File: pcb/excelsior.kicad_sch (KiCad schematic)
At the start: 10 parts, among them J1 USB_Hub4_FDD, J2 USB_Hub3, J3 USB_Hub2, J4 Conn_01x40_Socket, P1 Host_Port, P2 Left_Peripheral, P3 Right_Peripheral, U1 kb2040, U2 MCP23017_SO, U3 CH334R

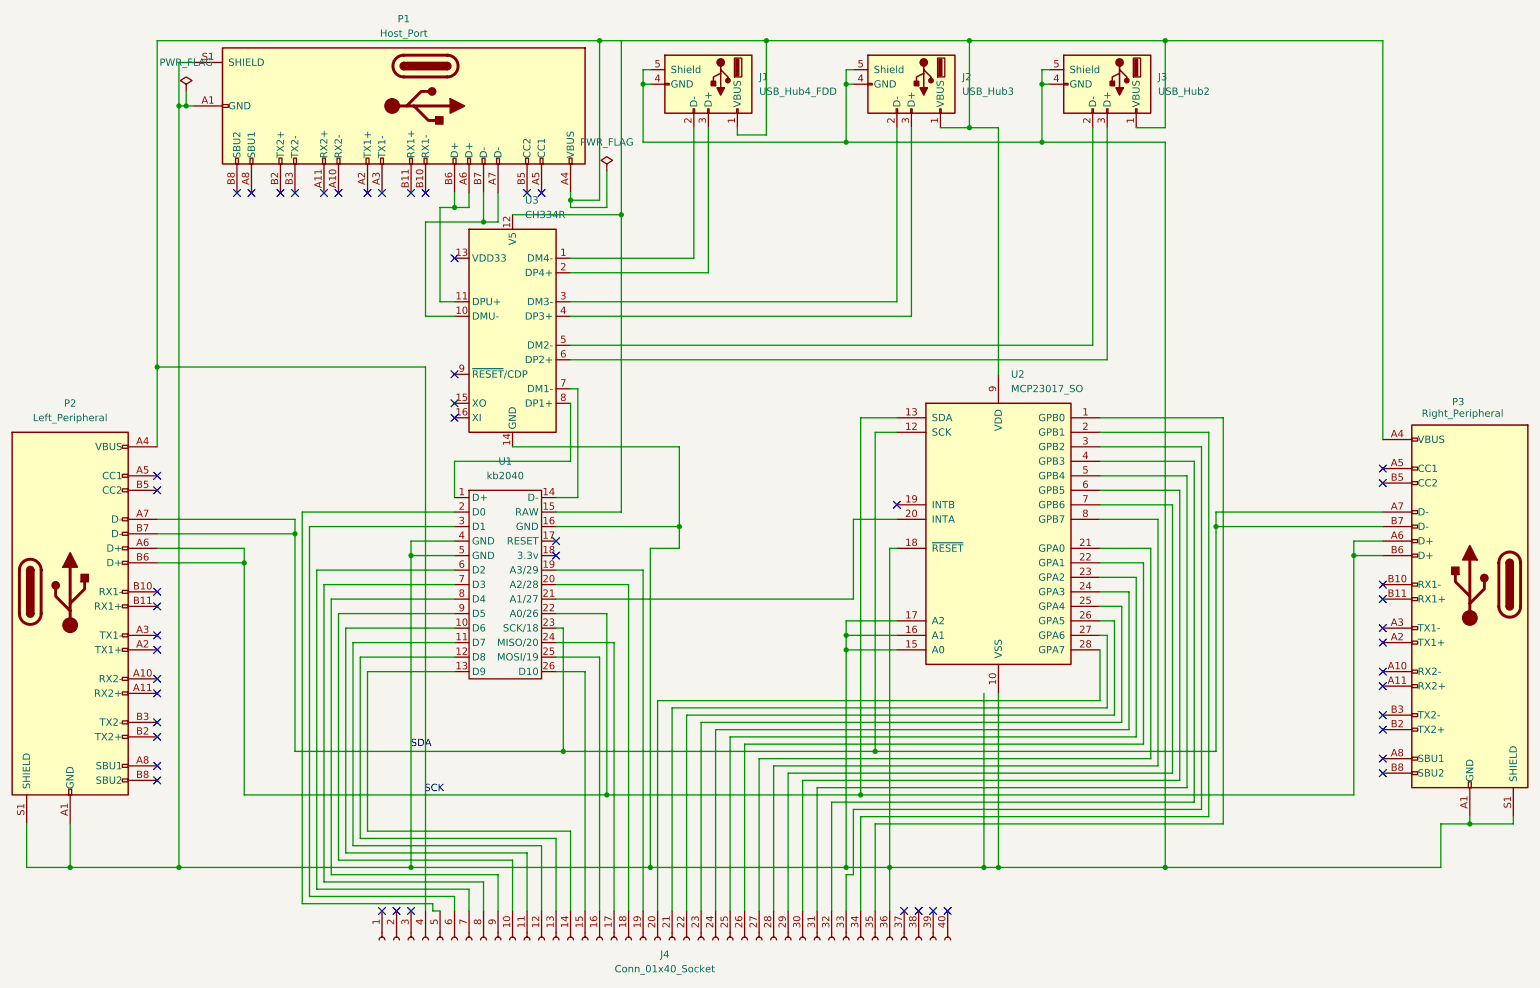
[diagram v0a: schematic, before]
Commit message: Continue work on PCB design.
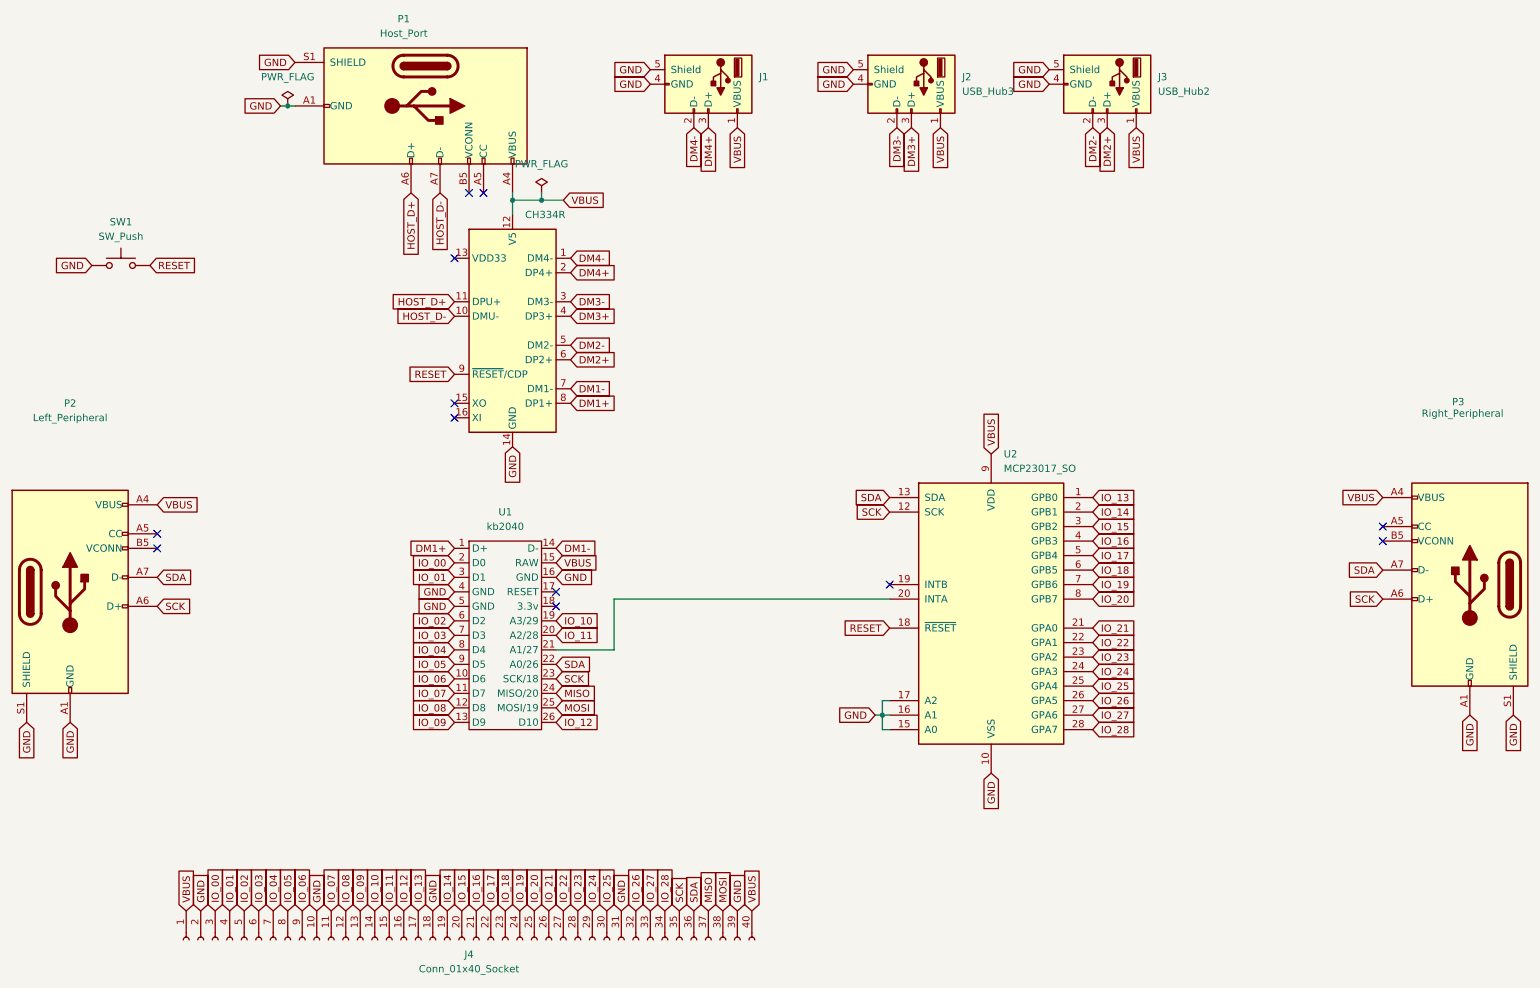
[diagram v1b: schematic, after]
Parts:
- added SW1: SW_Push, Button_Switch_SMD:SW_SPST_EVPBF, symbol Switch:SW_Push
- J1, J2, J3: footprint Connector_USB:USB_A_TE_292303-7_Horizontal -> Connector_USB:USB_A_Molex_67643_Horizontal
- P1, P2, P3: footprint Connector_USB:USB_C_Receptacle_Molex_105450-0101 -> Connector_USB:USB_C_Receptacle_GCT_USB4085; symbol Connector:USB_C_Receptacle -> Connector:USB_C_Plug_USB2.0
- U2: footprint Package_SO:SOIC-28W_7.5x17.9mm_P1.27mm -> Package_DIP:DIP-28_W7.62mm; symbol Interface_Expansion:MCP23017_SO -> Interface_Expansion:MCP23017_SP
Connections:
- net VBUS: now reaches J1.1 (VBUS), J2.1 (VBUS), J3.1 (VBUS), P1.A4 (VBUS), P1.A9 (VBUS), P1.B4 (VBUS), P1.B9 (VBUS), P2.A4 (VBUS), P2.A9 (VBUS), P2.B4 (VBUS), P2.B9 (VBUS), P3.A4 (VBUS), P3.A9 (VBUS), P3.B4 (VBUS), P3.B9 (VBUS), U1.15 (RAW), U2.9 (VDD), U3.12 (V5)
- net VBUS: now also J4.1 (Pin_1), J4.40 (Pin_40); no longer J4.4 (Pin_4)
- net DM2-: now reaches J3.2 (D-), U3.5 (DM2-)
- net DM2+: now reaches J3.3 (D+), U3.6 (DP2+)
- net GND: now reaches J1.4 (GND), J1.5 (Shield), J2.4 (GND), J2.5 (Shield), J3.4 (GND), J3.5 (Shield), P1.A1 (GND), P1.A12 (GND), P1.B1 (GND), P1.B12 (GND), P1.S1 (SHIELD), P2.A1 (GND), P2.A12 (GND), P2.B1 (GND), P2.B12 (GND), P2.S1 (SHIELD), P3.A1 (GND), P3.A12 (GND), P3.B1 (GND), P3.B12 (GND), P3.S1 (SHIELD), U1.16 (GND), U1.4 (GND), U1.5 (GND), U2.10 (VSS), U2.15 (A0), U2.16 (A1), U2.17 (A2), U3.14 (GND)
- net GND: now also J4.10 (Pin_10), J4.18 (Pin_18), J4.2 (Pin_2), J4.31 (Pin_31), J4.39 (Pin_39), SW1.1; no longer J4.36 (Pin_36), U2.18 (~{RESET})
- net IO_13: now reaches U2.1 (GPB0)
- net IO_13: now also J4.17 (Pin_17); no longer J4.35 (Pin_35)
- net IO_14: now reaches U2.2 (GPB1)
- net IO_14: now also J4.19 (Pin_19); no longer J4.34 (Pin_34)
- net IO_21: now reaches U2.21 (GPA0)
- net IO_21: now also J4.26 (Pin_26); no longer J4.27 (Pin_27)
- net IO_22: now reaches U2.22 (GPA1)
- net IO_22: now also J4.27 (Pin_27); no longer J4.26 (Pin_26)
- net IO_20: now reaches J4.25 (Pin_25)
- net IO_20: now also U2.8 (GPB7); no longer U2.23 (GPA2)
- net IO_19: now reaches J4.24 (Pin_24)
- net IO_19: now also U2.7 (GPB6); no longer U2.24 (GPA3)
- net IO_18: now reaches J4.23 (Pin_23)
- net IO_18: now also U2.6 (GPB5); no longer U2.25 (GPA4)
- net IO_17: now reaches J4.22 (Pin_22)
- net IO_17: now also U2.5 (GPB4); no longer U2.26 (GPA5)
- net IO_16: now reaches J4.21 (Pin_21)
- net IO_16: now also U2.4 (GPB3); no longer U2.27 (GPA6)
- net IO_15: now reaches J4.20 (Pin_20)
- net IO_15: now also U2.3 (GPB2); no longer U2.28 (GPA7)
- net IO_27: now reaches J4.33 (Pin_33)
- net IO_27: now also U2.27 (GPA6); no longer U2.3 (GPB2)
- net IO_26: now reaches J4.32 (Pin_32)
- net IO_26: now also U2.26 (GPA5); no longer U2.4 (GPB3)
- net IO_25: now reaches J4.30 (Pin_30)
- net IO_25: now also U2.25 (GPA4); no longer U2.6 (GPB5)
- net IO_24: now reaches J4.29 (Pin_29)
- net IO_24: now also U2.24 (GPA3); no longer U2.7 (GPB6)
- net IO_23: now reaches J4.28 (Pin_28)
- net IO_23: now also U2.23 (GPA2); no longer U2.8 (GPB7)
- net DM4-: now reaches J1.2 (D-), U3.1 (DM4-)
- net HOST_D-: now reaches P1.A7 (D-), U3.10 (DMU-)
- net HOST_D-: no longer P1.B7 (D-)
- net HOST_D+: now reaches P1.A6 (D+), U3.11 (DPU+)
- net HOST_D+: no longer P1.B6 (D+)
- net DM4+: now reaches J1.3 (D+), U3.2 (DP4+)
- net DM3-: now reaches J2.2 (D-), U3.3 (DM3-)
- net DM3+: now reaches J2.3 (D+), U3.4 (DP3+)
- net DM1-: now reaches U1.14 (D-), U3.7 (DM1-)
- net DM1+: now reaches U1.1 (D+), U3.8 (DP1+)
- net RESET: now reaches U3.9 (~{RESET}/CDP)
- net RESET: now also U2.18 (~{RESET}), SW1.2
- net IO_06: now reaches U1.10 (D6)
- net IO_06: now also J4.9 (Pin_9); no longer J4.11 (Pin_11)
- net IO_07: now reaches U1.11 (D7)
- net IO_07: now also J4.11 (Pin_11); no longer J4.12 (Pin_12)
- net IO_08: now reaches U1.12 (D8)
- net IO_08: now also J4.12 (Pin_12); no longer J4.13 (Pin_13)
- net IO_09: now reaches U1.13 (D9)
- net IO_09: now also J4.13 (Pin_13); no longer J4.14 (Pin_14)
- net IO_10: now reaches U1.19 (A3/29)
- net IO_10: now also J4.14 (Pin_14); no longer J4.19 (Pin_19)
- net IO_00: now reaches U1.2 (D0)
- net IO_00: now also J4.3 (Pin_3); no longer J4.5 (Pin_5)
- net IO_11: now reaches U1.20 (A2/28)
- net IO_11: now also J4.15 (Pin_15); no longer J4.18 (Pin_18)
- net MISO: now reaches U1.24 (MISO/20)
- net MISO: now also J4.37 (Pin_37); no longer J4.17 (Pin_17)
- net IO_12: now reaches J4.16 (Pin_16)
- net IO_12: now also U1.26 (D10); no longer U1.25 (MOSI/19)
- net IO_01: now reaches U1.3 (D1)
- net IO_01: now also J4.4 (Pin_4); no longer J4.6 (Pin_6)
- net IO_02: now reaches U1.6 (D2)
- net IO_02: now also J4.5 (Pin_5); no longer J4.7 (Pin_7)
- net IO_03: now reaches U1.7 (D3)
- net IO_03: now also J4.6 (Pin_6); no longer J4.8 (Pin_8)
- net IO_04: now reaches U1.8 (D4)
- net IO_04: now also J4.7 (Pin_7); no longer J4.9 (Pin_9)
- net IO_05: now reaches U1.9 (D5)
- net IO_05: now also J4.8 (Pin_8); no longer J4.10 (Pin_10)
- net MOSI: now reaches J4.38 (Pin_38)
- net MOSI: now also U1.25 (MOSI/19)
- new net IO_28: J4.34 (Pin_34), U2.28 (GPA7)
- new net SCK: J4.35 (Pin_35), P2.A6 (D+), P3.A6 (D+), U1.23 (SCK/18), U2.12 (SCK)
- new net SDA: J4.36 (Pin_36), P2.A7 (D-), P3.A7 (D-), U1.22 (A0/26), U2.13 (SDA)
- no-connect marks 50 -> 12
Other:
- note removed: "SCK"
- note removed: "SDA"
- moved on the sheet: J4, U1, U2

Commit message: Continue work on PCBs, add Gerber files.
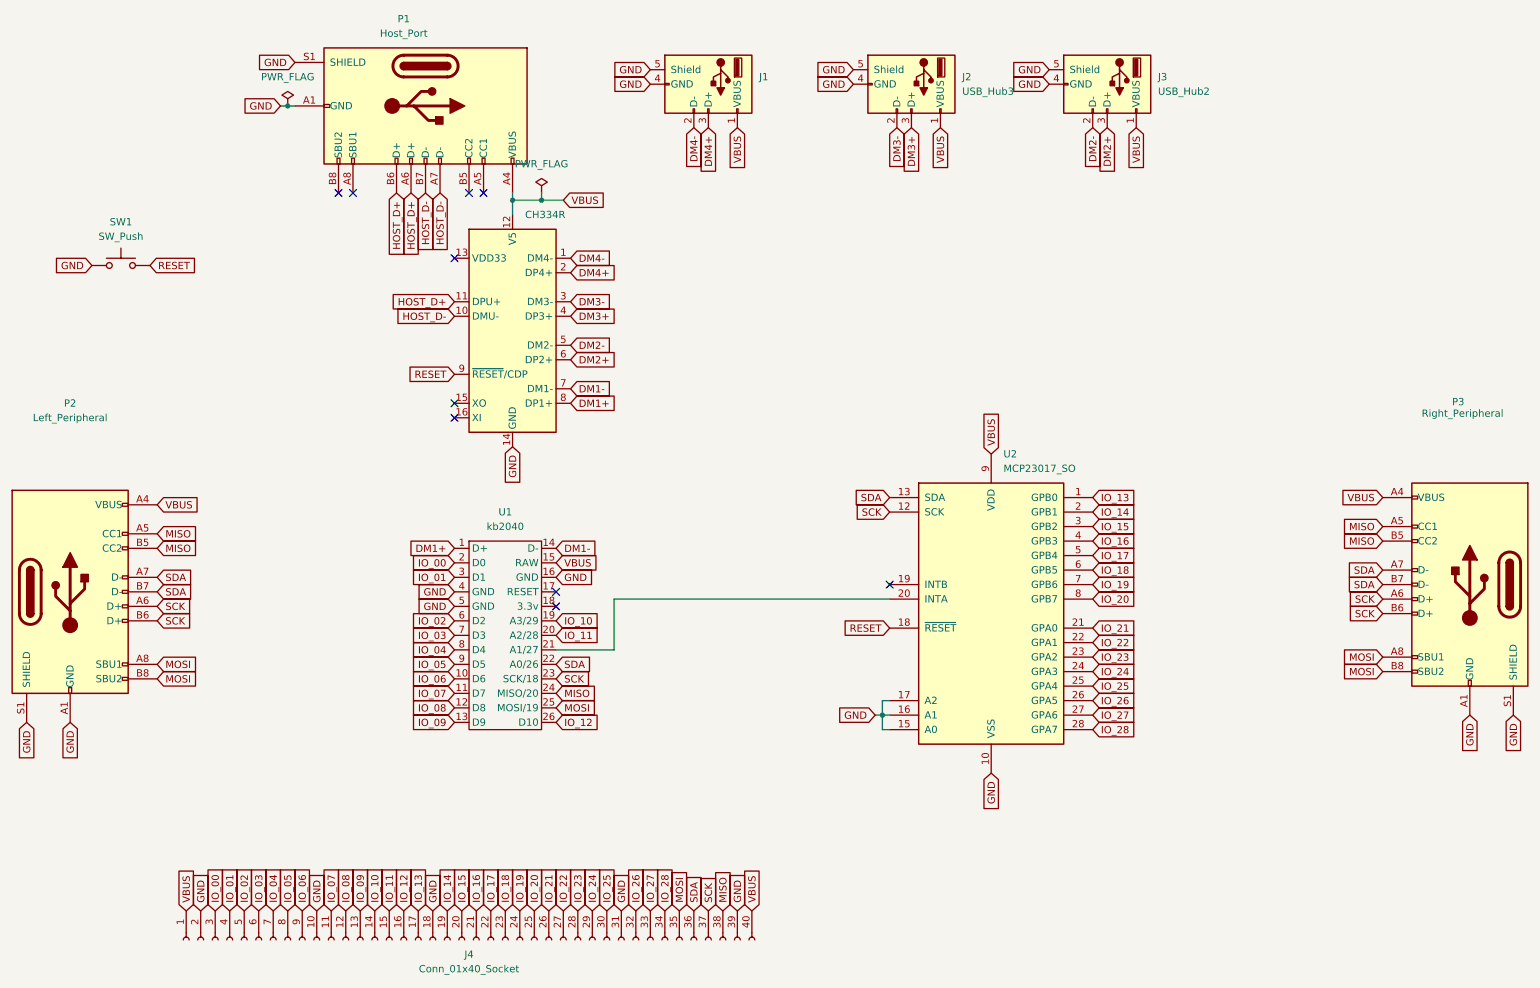
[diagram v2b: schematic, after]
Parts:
- P1, P2, P3: symbol Connector:USB_C_Plug_USB2.0 -> Connector:USB_C_Receptacle_USB2.0_16P
- U2: footprint Package_DIP:DIP-28_W7.62mm -> Package_SO:SOIC-28W_7.5x17.9mm_P1.27mm; symbol Interface_Expansion:MCP23017_SP -> Interface_Expansion:MCP23017_SO
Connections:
- net HOST_D+: now also P1.B6 (D+)
- net HOST_D-: now also P1.B7 (D-)
- net MISO: now also J4.38 (Pin_38), P2.A5 (CC1), P2.B5 (CC2), P3.A5 (CC1), P3.B5 (CC2); no longer J4.37 (Pin_37)
- net MOSI: now also J4.35 (Pin_35), P2.A8 (SBU1), P2.B8 (SBU2), P3.A8 (SBU1), P3.B8 (SBU2); no longer J4.38 (Pin_38)
- net SCK: now also J4.37 (Pin_37), P2.B6 (D+), P3.B6 (D+); no longer J4.35 (Pin_35)
- net SDA: now also P2.B7 (D-), P3.B7 (D-)
- no-connect marks 12 -> 10

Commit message: Continue work on PCBs, add gitignore and remove backup files.
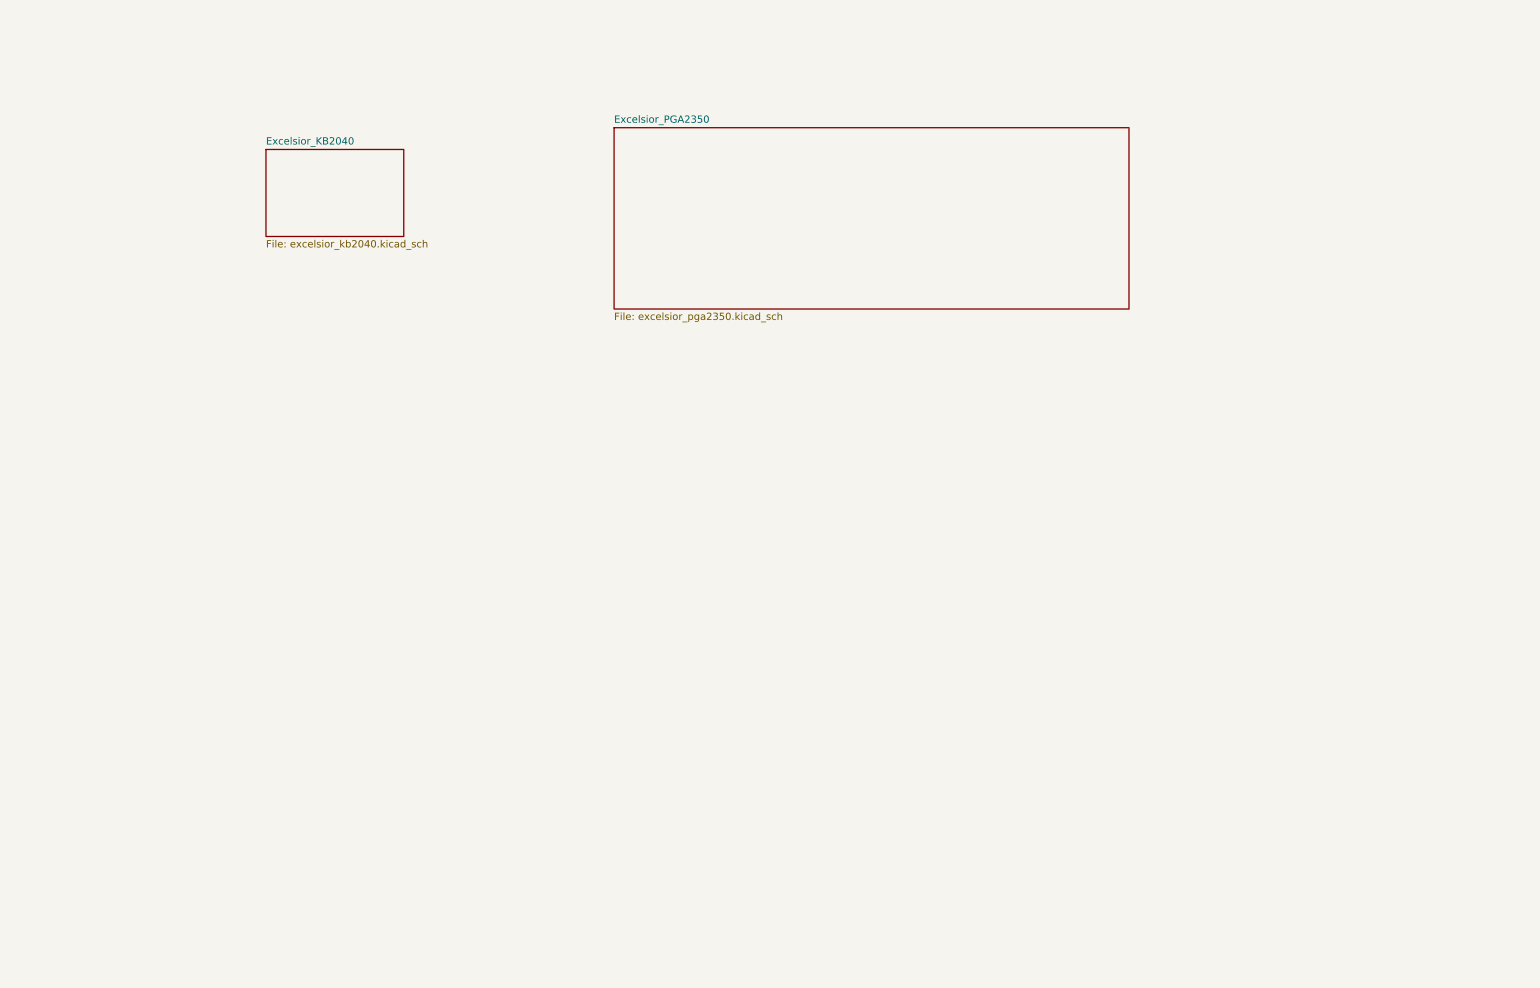
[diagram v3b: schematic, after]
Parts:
- removed J1: USB_Hub4_FDD, Connector_USB:USB_A_Molex_67643_Horizontal, symbol Connector:USB_A
- removed J2: USB_Hub3, Connector_USB:USB_A_Molex_67643_Horizontal, symbol Connector:USB_A
- removed J3: USB_Hub2, Connector_USB:USB_A_Molex_67643_Horizontal, symbol Connector:USB_A
- removed J4: Conn_01x40_Socket, Connector_PinHeader_2.54mm:PinHeader_1x40_P2.54mm_Vertical, symbol Connector:Conn_01x40_Socket
- removed P1: Host_Port, Connector_USB:USB_C_Receptacle_GCT_USB4085, symbol Connector:USB_C_Receptacle_USB2.0_16P
- removed P2: Left_Peripheral, Connector_USB:USB_C_Receptacle_GCT_USB4085, symbol Connector:USB_C_Receptacle_USB2.0_16P
- removed P3: Right_Peripheral, Connector_USB:USB_C_Receptacle_GCT_USB4085, symbol Connector:USB_C_Receptacle_USB2.0_16P
- removed SW1: SW_Push, Button_Switch_SMD:SW_SPST_EVPBF, symbol Switch:SW_Push
- removed U1: kb2040, footprints:kb2040, symbol kb2040:kb2040
- removed U2: MCP23017_SO, Package_SO:SOIC-28W_7.5x17.9mm_P1.27mm, symbol Interface_Expansion:MCP23017_SO
- removed U3: CH334R, Package_SO:QSOP-16_3.9x4.9mm_P0.635mm, symbol Interface_USB:CH334R
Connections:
- no-connect marks 10 -> 0
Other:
- added sheet Excelsior_KB2040 (excelsior_kb2040.kicad_sch)
- added sheet Excelsior_PGA2350 (excelsior_pga2350.kicad_sch)

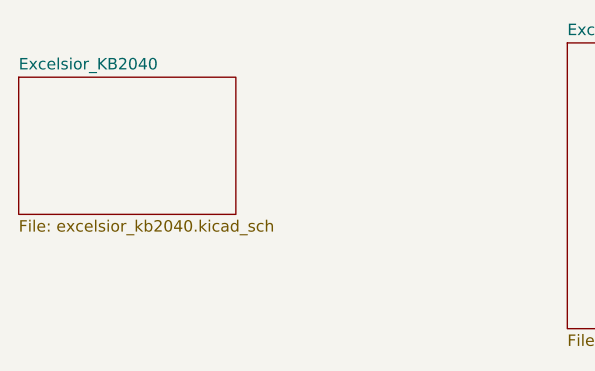
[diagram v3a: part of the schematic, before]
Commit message: Continue work on PCBs.
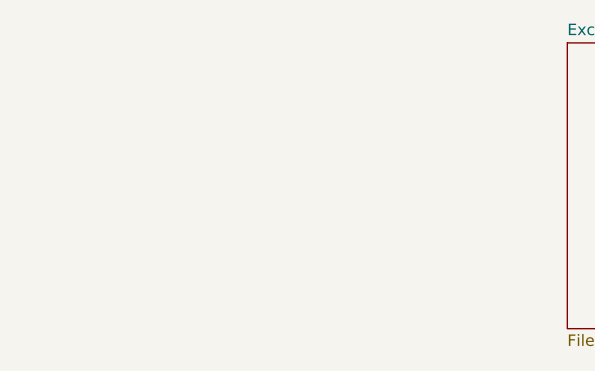
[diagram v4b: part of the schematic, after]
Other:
- removed sheet Excelsior_KB2040
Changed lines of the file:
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@@
 	(paper "A4")
-	(sheet
-		(at 59.69 39.37)
-		(size 24.13 15.24)
-		(exclude_from_sim no)
-		(in_bom yes)
-		(on_board yes)
-		(dnp no)
-		(fields_autoplaced yes)
-		(stroke
-			(width 0.1524)
-			(type solid)
-		)
-		(fill
-			(color 0 0 0 0.0000)
-		)
-		(property "Sheetname" "Excelsior_KB2040"
-			(at 59.69 38.6584 0)
-			(effects
-				(font
-					(size 1.27 1.27)
-				)
-				(justify left bottom)
-			)
-		)
-		(property "Sheetfile" "excelsior_kb2040.kicad_sch"
-			(at 59.69 55.1946 0)
-			(effects
-				(font
-					(size 1.27 1.27)
-				)
-				(justify left top)
-			)
-		)
-		(instances
-			(project "excelsior"
-				(path "/68aab48b-d026-4610-86b4-a3277e874325"
-					(page "3")
-				)
-			)
-		)
-	)
 	(sheet
 		(at 120.65 35.56)
